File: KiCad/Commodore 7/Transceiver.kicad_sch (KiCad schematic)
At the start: 1 part, among them U7 SN65HVD74DR

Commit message: uhhhhhhhh idk
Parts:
- U7: footprint D8_TEX -> 2N65HVD74DR:D8_TEX
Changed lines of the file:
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@@
 			)
 		)
-		(property "Footprint" "D8_TEX"
+		(property "Footprint" "2N65HVD74DR:D8_TEX"
 			(at 40.64 44.45 0)
 			(effects

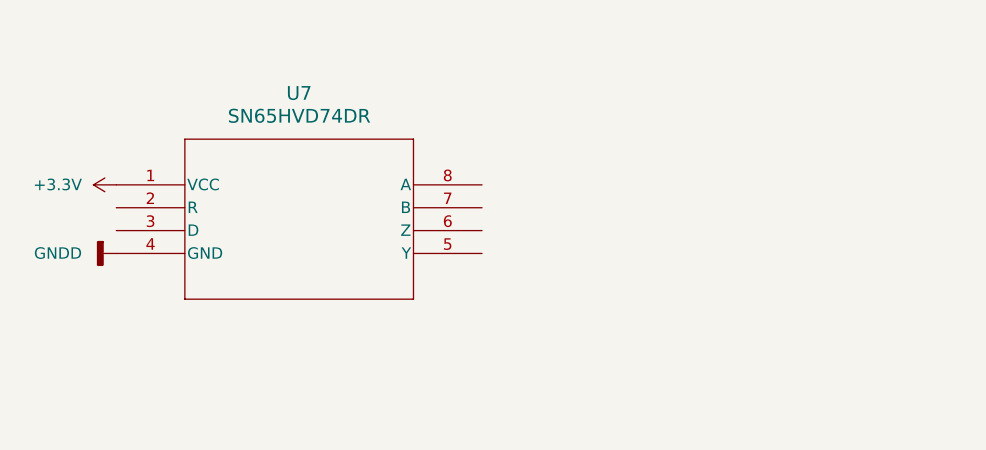
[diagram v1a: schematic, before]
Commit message: i sitll got mroe to do ssry yall
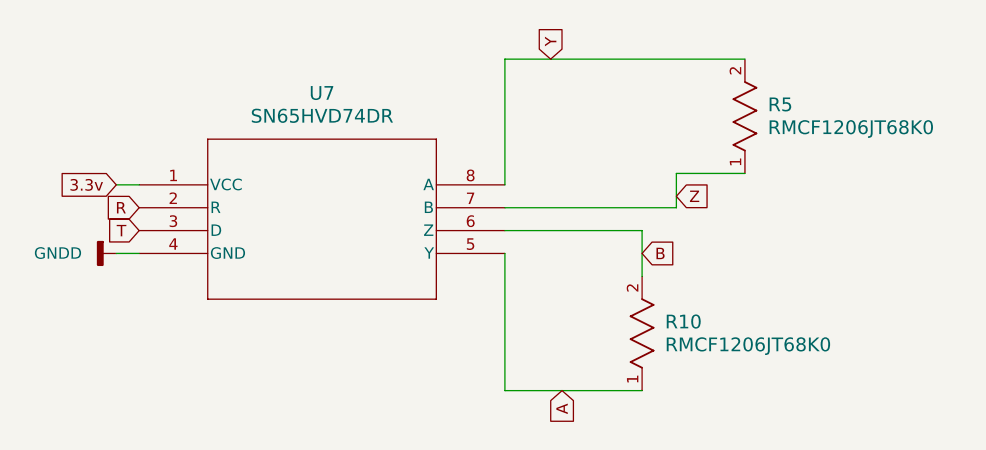
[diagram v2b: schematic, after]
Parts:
- added R10, R5: RMCF1206JT68K0, Resistor_SMD:R_1206_3216Metric, symbol RMCF1206JT68K0:RMCF1206JT68K0
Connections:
- net R: now reaches U7.2 (R)
- net T: now reaches U7.3 (D)
- net A: now reaches U7.5 (Y)
- net A: now also R10.1
- net B: now reaches U7.6 (Z)
- net B: now also R10.2
- net Z: now reaches U7.7 (B)
- net Z: now also R5.1
- net Y: now reaches U7.8 (A)
- net Y: now also R5.2
- net +3.3V renamed 3.3v
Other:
- moved on the sheet: U7
